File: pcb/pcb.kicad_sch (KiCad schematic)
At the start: 4 parts

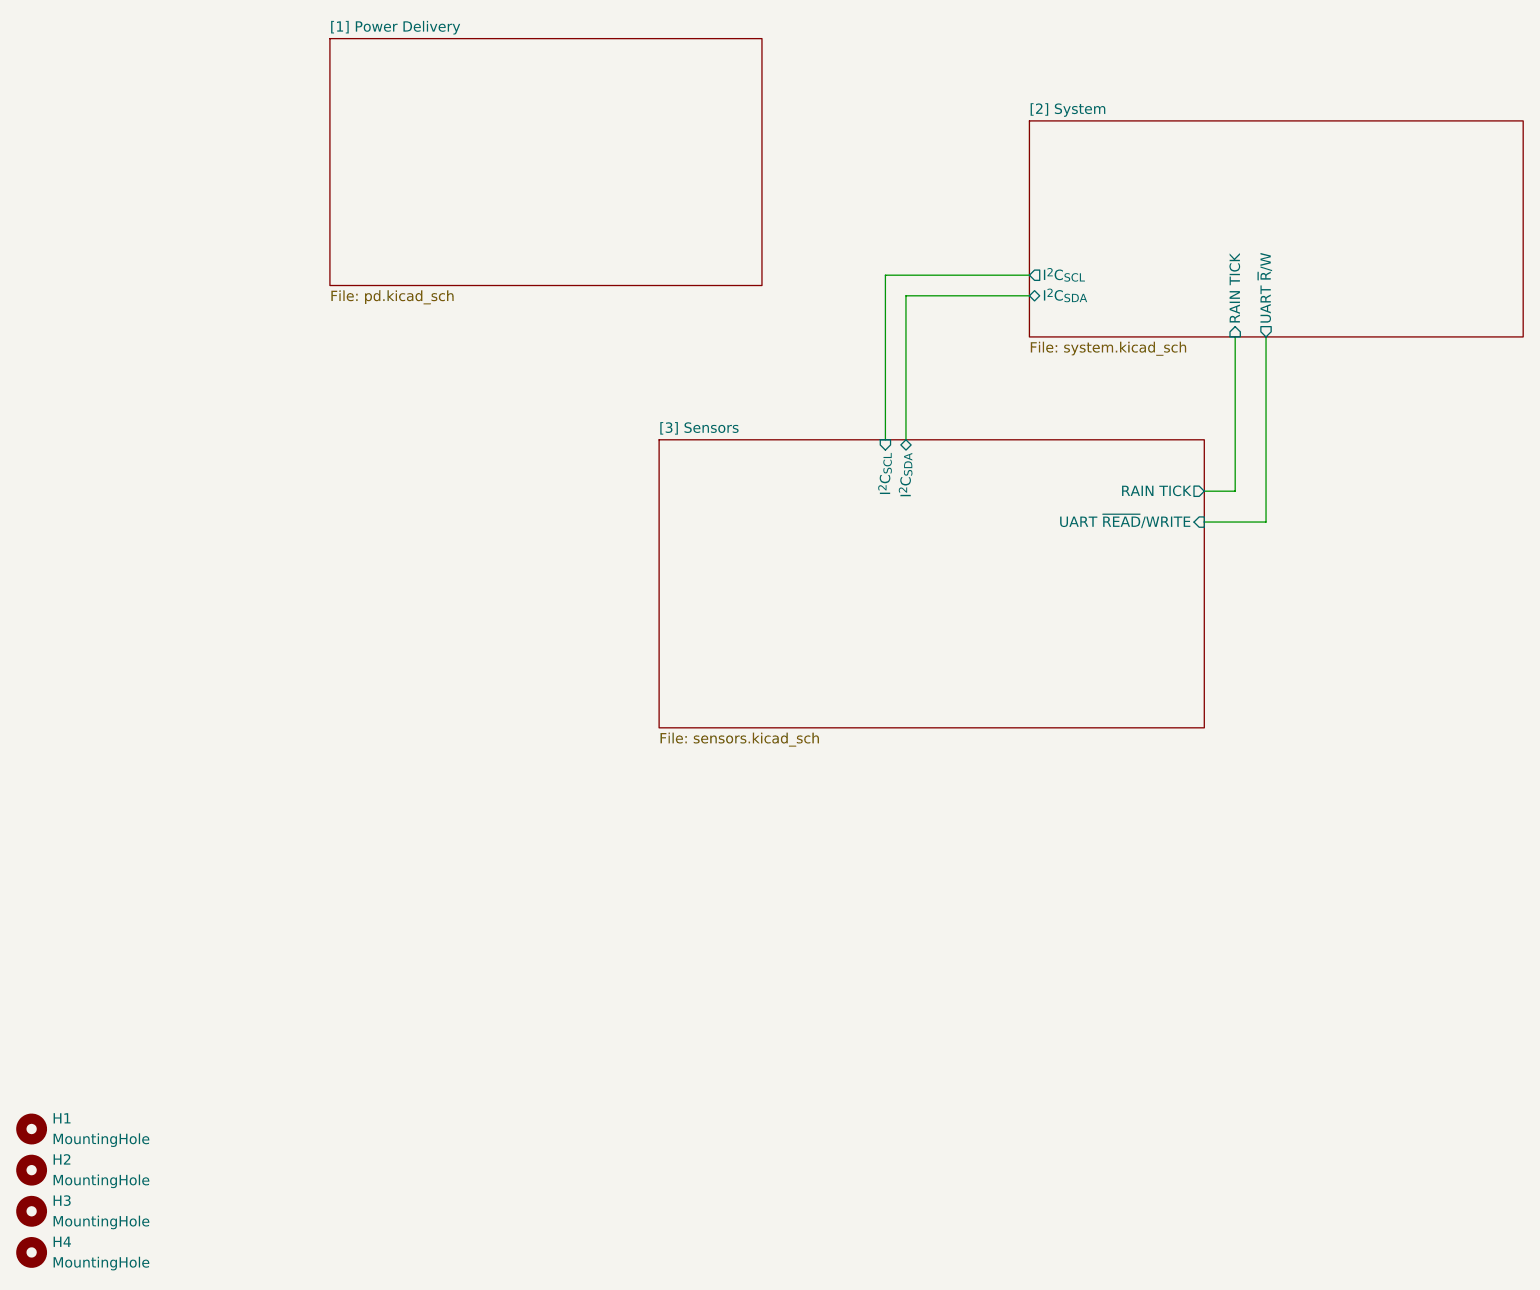
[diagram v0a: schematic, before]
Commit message: feat: wiring
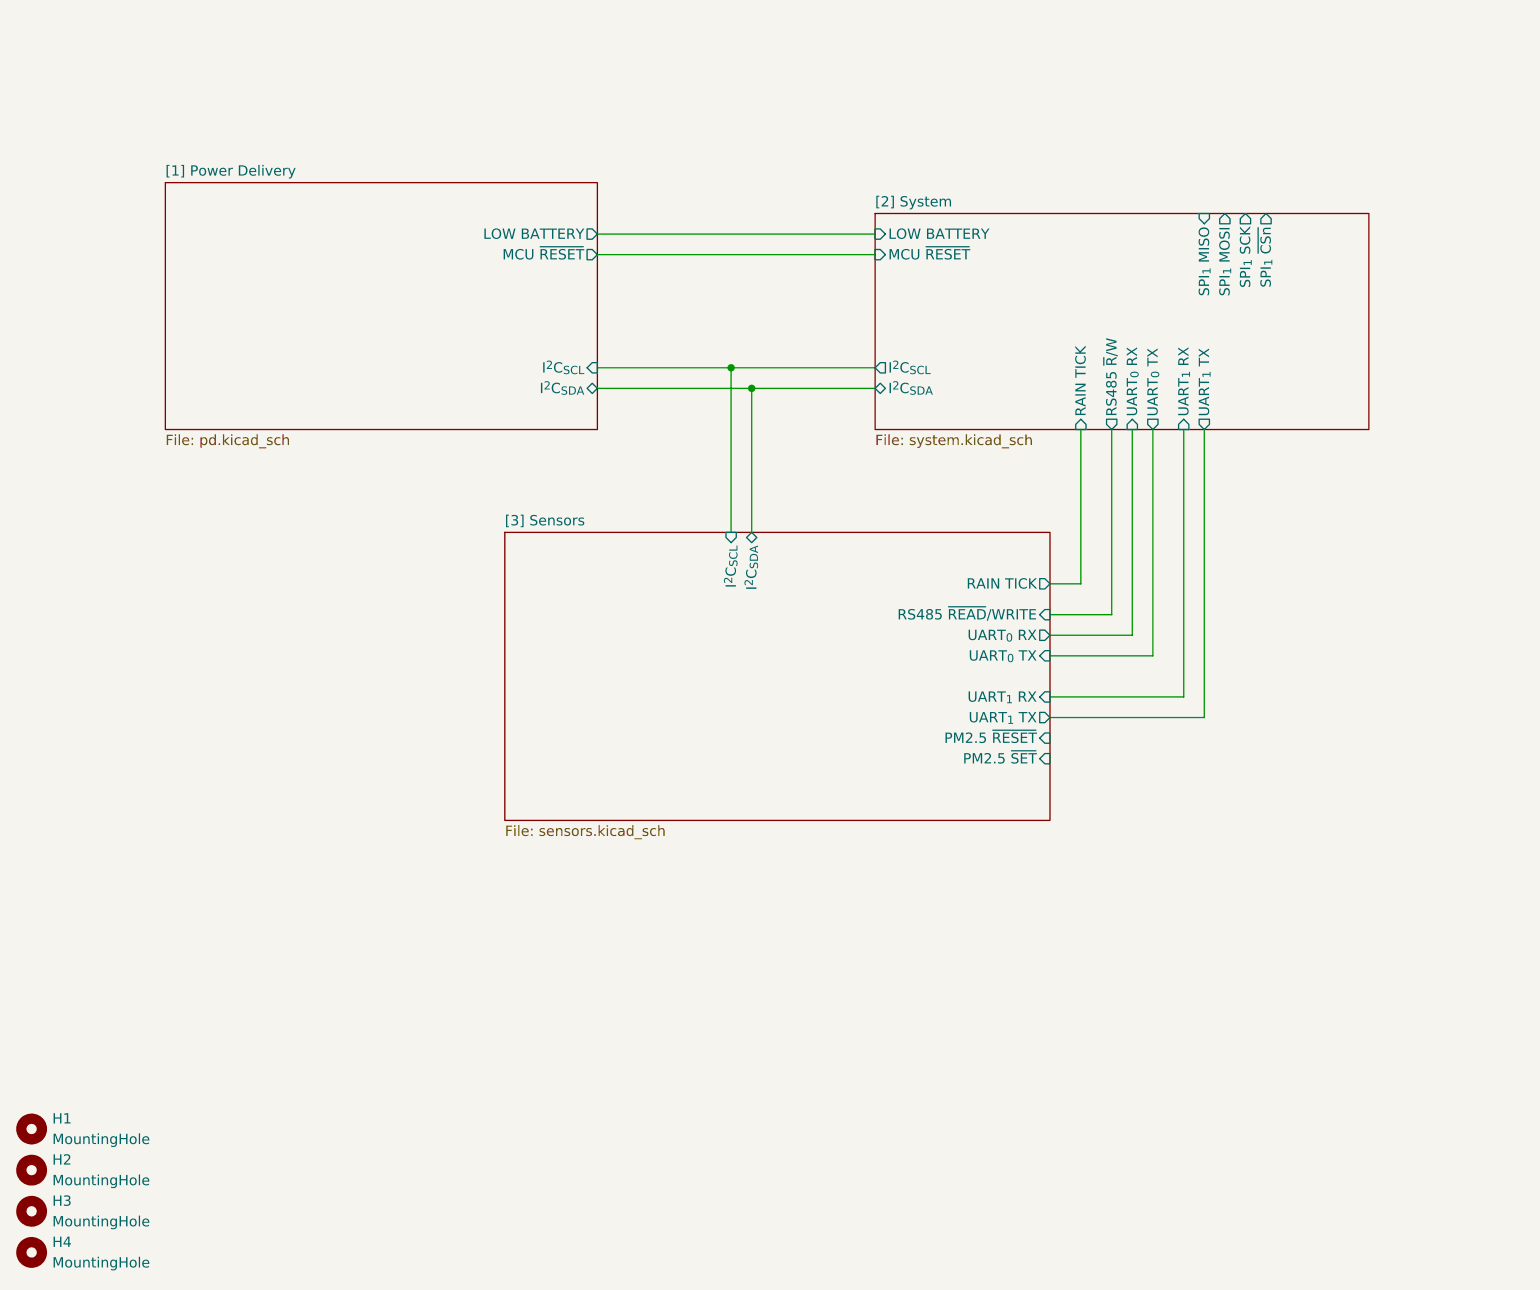
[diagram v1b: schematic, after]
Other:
- sheet [1] Power Delivery ports: added I^{2}C_{SCL}, I^{2}C_{SDA}, LOW BATTERY, MCU ~{RESET}; removed none
- sheet [2] System ports: added LOW BATTERY, MCU ~{RESET}, RS485 ~{R}/W, SPI_{1} MISO, SPI_{1} MOSI, SPI_{1} SCK, SPI_{1} ~{CSn}, UART_{0} RX, UART_{0} TX, UART_{1} RX, UART_{1} TX; removed UART ~{R}/W
- sheet [3] Sensors ports: added PM2.5 ~{RESET}, PM2.5 ~{SET}, RS485 ~{READ}/WRITE, UART_{0} RX, UART_{0} TX, UART_{1} RX, UART_{1} TX; removed UART ~{READ}/WRITE
